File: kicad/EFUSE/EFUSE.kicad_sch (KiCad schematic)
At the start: 17 parts, among them J1 Input, J2 Output, Q1 Si7336ADP, U1 LTC4215IUFD-1_PBF

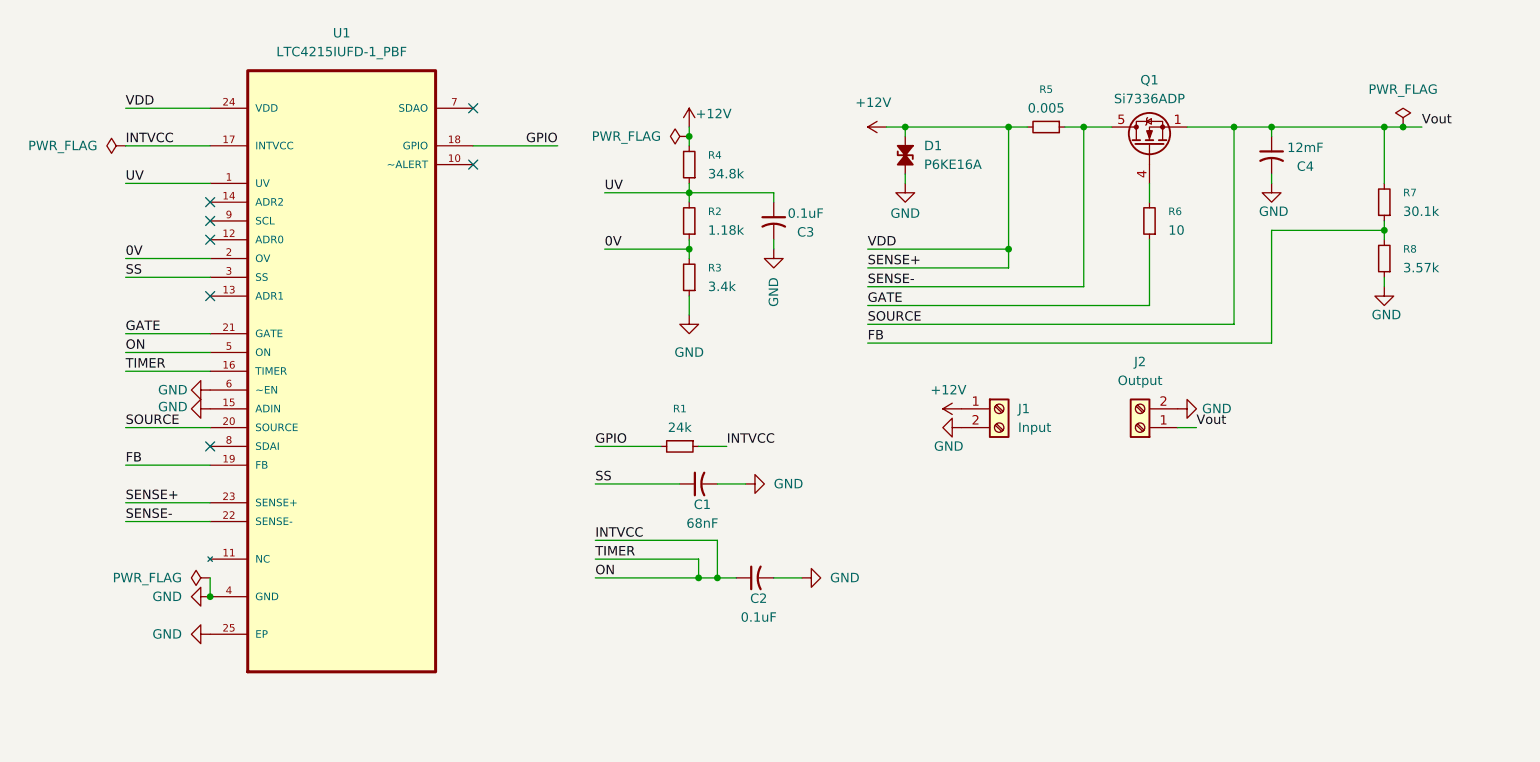
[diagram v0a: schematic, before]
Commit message: Change on Image
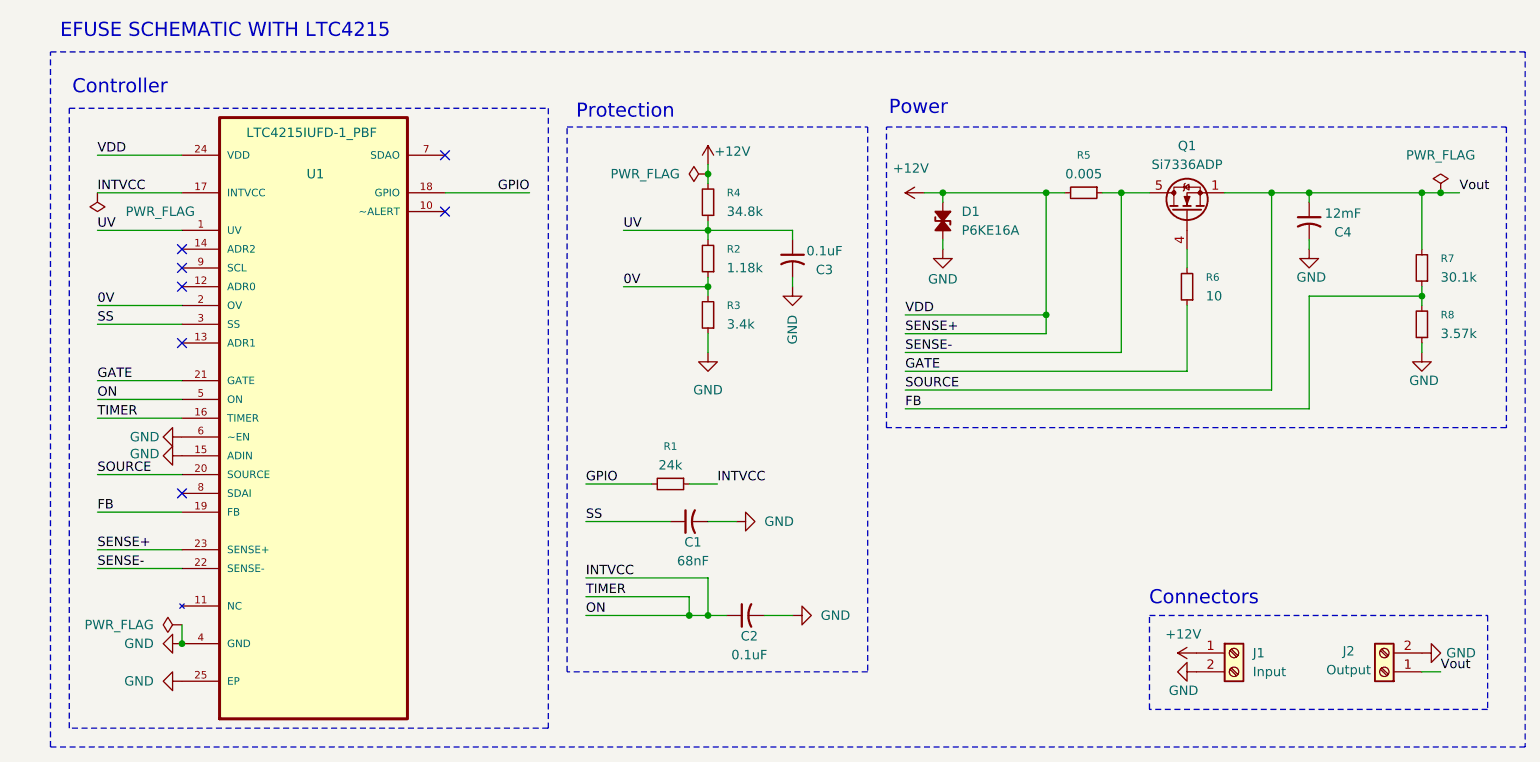
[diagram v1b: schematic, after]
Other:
- note added: "Connectors"
- note added: "Controller"
- note added: "EFUSE SCHEMATIC WITH LTC4215"
- note added: "Power"
- note added: "Protection"
- moved on the sheet: C1, C2, C3, C4, D1, J1, J2, Q1, R1, R2, R3, R4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
